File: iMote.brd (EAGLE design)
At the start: 50 x 50 mm, 47 parts, among them CN1 C-02235, CN2 ICSP, CN3 CC-HEADER, IC1 ATmega328P-AU, IC2 FT232RLSSOP, IC3 BLE112-A-VISUAL, Q1 16MHz, T1 2SC1815

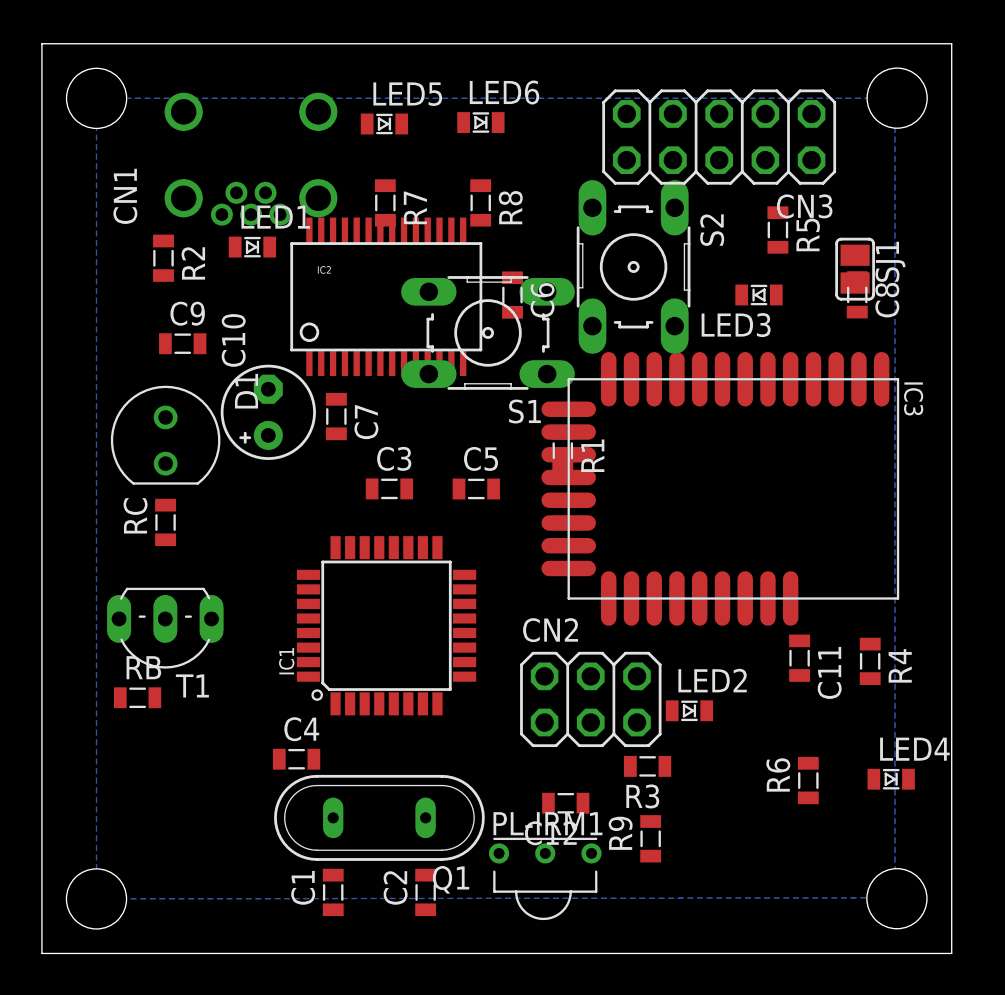
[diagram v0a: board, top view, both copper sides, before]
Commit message: 5cmx5cmにおさまった!
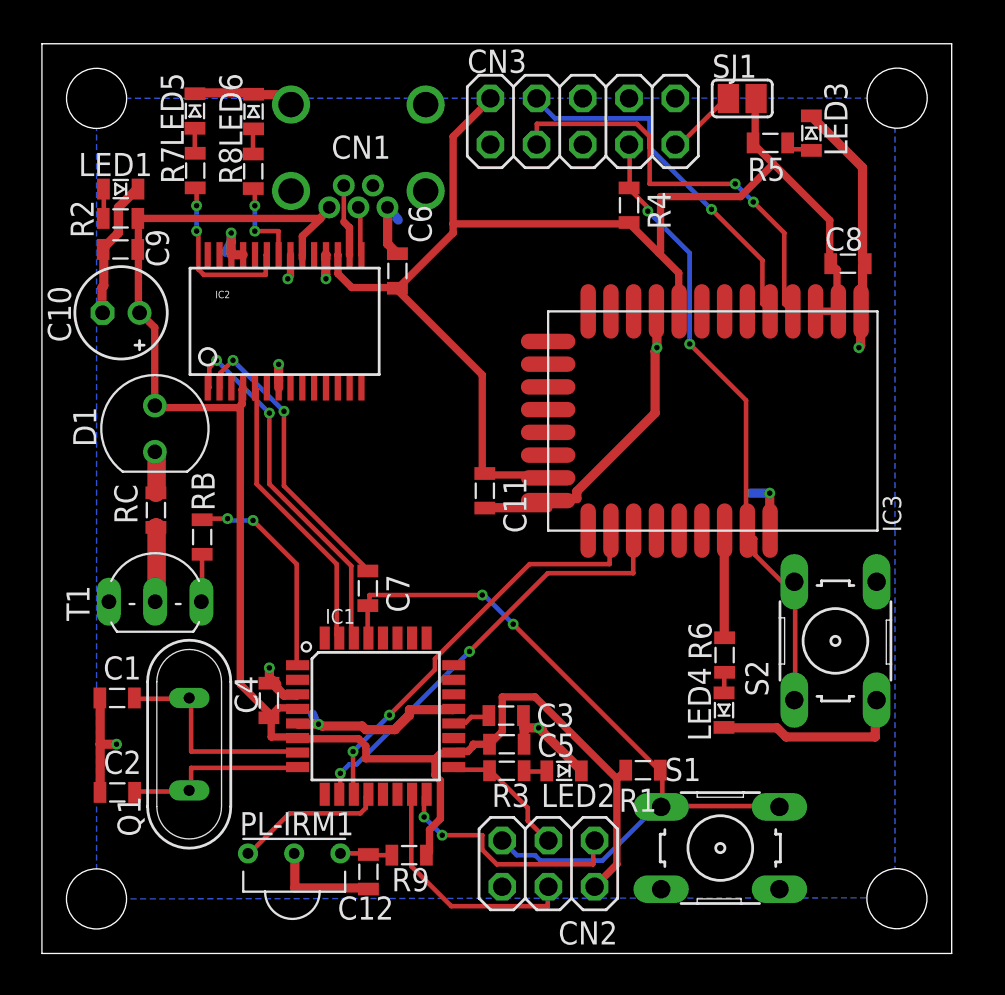
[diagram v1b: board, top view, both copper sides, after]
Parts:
- C10: device rcl:E2,5-5 -> my:E2-5
- moved S1 31.1 mm to (37.3, 5.79), turned to 0 degrees
- moved R4 28.4 mm to (32.3, 41.1)
- moved S2 23.4 mm to (43.6, 17.2), turned to 90 degrees
- moved C11 19.6 mm to (24.3, 25.4)
- moved R1 18.1 mm to (33.0, 10.1), turned to 180 degrees
- moved C2 17.8 mm to (4.14, 8.85), turned to 0 degrees
- moved C1 16.0 mm to (4.13, 14.0), turned to 0 degrees
- moved C5 14.1 mm to (25.5, 11.5), turned to 180 degrees
- moved C3 14.0 mm to (25.5, 13.1), turned to 180 degrees
- moved PL-IRM1 13.8 mm to (13.9, 5.50)
- moved R9 13.3 mm to (20.2, 5.40), turned to 0 degrees
- moved R8 12.6 mm to (11.6, 43.0)
- moved LED6 12.5 mm to (11.6, 46.3), turned to 90 degrees
- moved C12 11.5 mm to (17.9, 4.49), turned to 270 degrees
- moved SJ1 11.2 mm to (38.5, 47.0), turned to 0 degrees
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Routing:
- net GND: track 0.00 -> 101.4 mm, vias 0 -> 11
- net +5V: track 0.00 -> 88.7 mm
- net +3V3: track 0.00 -> 73.9 mm
- net !RESET: track 0.00 -> 41.4 mm, vias 0 -> 2
- net !BLE/RST: track 0.00 -> 35.6 mm, vias 0 -> 2
- net D6/BLERX: track 0.00 -> 24.2 mm, vias 0 -> 2
- net BLE/P2_2: track 0.00 -> 23.3 mm, vias 0 -> 2
- net D7/BLETX: track 0.00 -> 23.0 mm, vias 0 -> 2
- net D0/USBRX: track 0.00 -> 20.1 mm, vias 0 -> 2
- net BLE/P2_1: track 0.00 -> 20.1 mm, vias 0 -> 1
- net N$8: track 0.00 -> 16.5 mm, vias 0 -> 2
- net D1/USBTX: track 0.00 -> 15.7 mm
- net D12/MISO: track 0.00 -> 13.5 mm, vias 0 -> 2
- net D11/MOSI: track 0.00 -> 13.5 mm
- net N$2: track 0.00 -> 11.9 mm
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
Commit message: いい感じや
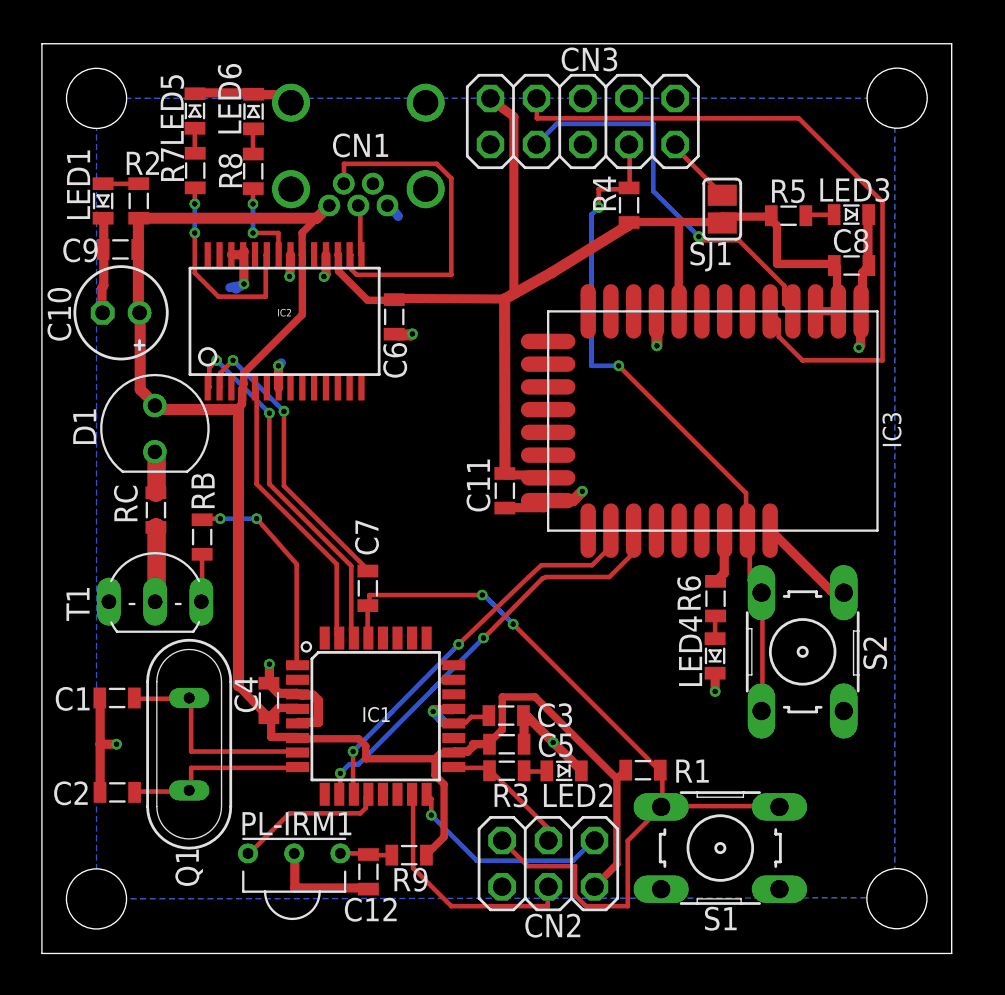
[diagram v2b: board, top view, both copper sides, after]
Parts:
- moved SJ1 6.18 mm to (37.4, 40.9), turned to 270 degrees
- moved LED3 4.99 mm to (44.5, 40.6), turned to 0 degrees
- moved R5 4.12 mm to (41.0, 40.5)
- moved R6 3.14 mm to (37.0, 19.5)
- moved LED4 3.02 mm to (37.0, 16.4)
- moved C6 2.53 mm to (19.4, 35.0), turned to 270 degrees
- moved S2 1.90 mm to (41.8, 16.6)
- moved R2 1.39 mm to (5.32, 41.4), turned to 90 degrees
- moved LED1 1.17 mm to (3.36, 41.4), turned to 270 degrees
- moved C11 1.10 mm to (25.4, 25.4)
- moved C8 0.22 mm to (44.5, 37.8)
- moved CN1 0.10 mm to (17.4, 44.5)
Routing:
- net GND: track 101.4 -> 70.0 mm, vias 11 -> 13
- net BLE/P2_1: track 20.1 -> 38.5 mm, vias 1 -> 0
- net USBD-: track 3.94 -> 19.1 mm
- net +5V: track 88.7 -> 97.5 mm
- net +3V3: track 73.9 -> 65.9 mm
- net !RESET: track 41.4 -> 46.5 mm
- net BLE/P0_0: track 5.90 -> 3.00 mm
- net !BLE/RST: track 35.6 -> 37.8 mm
- net USB/TXLED: track 9.54 -> 11.5 mm
- net D12/MISO: track 13.5 -> 11.7 mm, vias 2 -> 1
- net BLE/P2_2: track 23.3 -> 21.7 mm, vias 2 -> 1
- net D7/BLETX: track 23.0 -> 22.3 mm
